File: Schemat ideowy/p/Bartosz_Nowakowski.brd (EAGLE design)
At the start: 41.6 x 33.5 mm, 23 parts, among them J2 6_PIN_SERIAL_CABLEPTH, U1 ESP8266, U2 4MB Flash, Y1 CRYSTAL-26MHZSMD-3.2X2.5

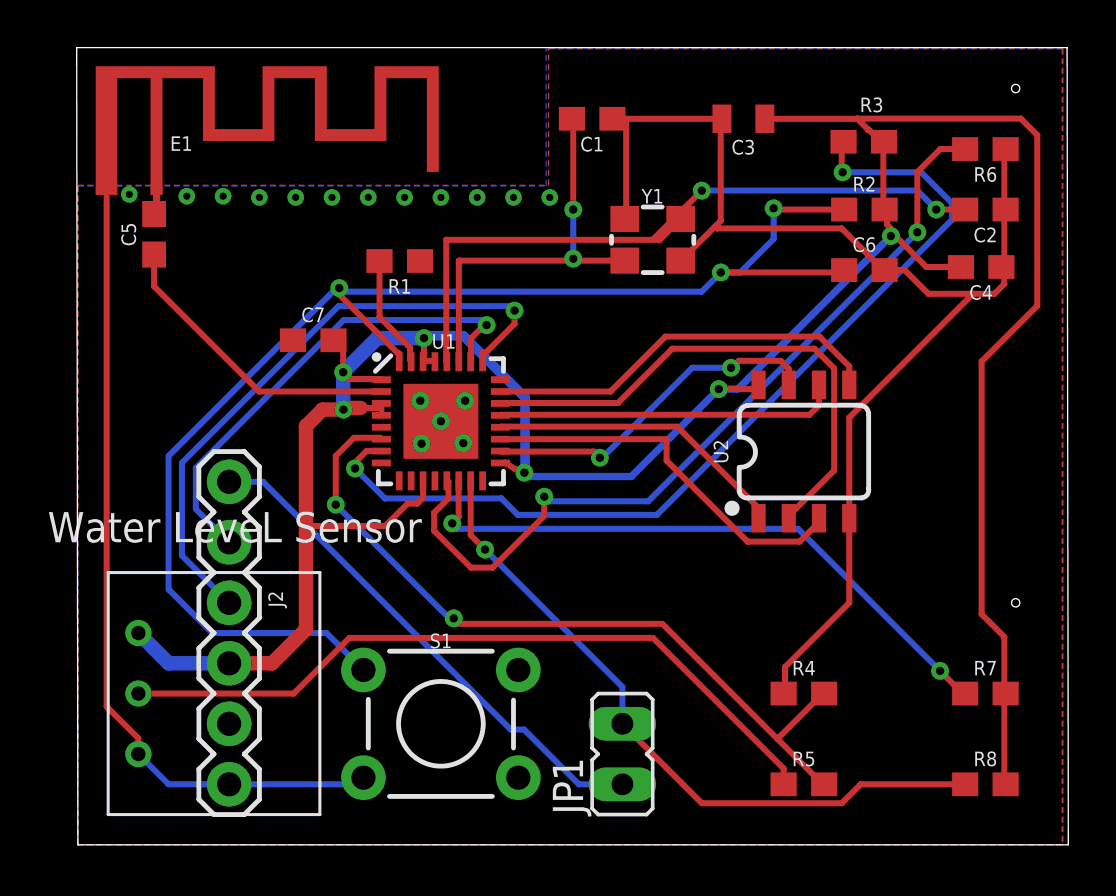
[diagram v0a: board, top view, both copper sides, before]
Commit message: update
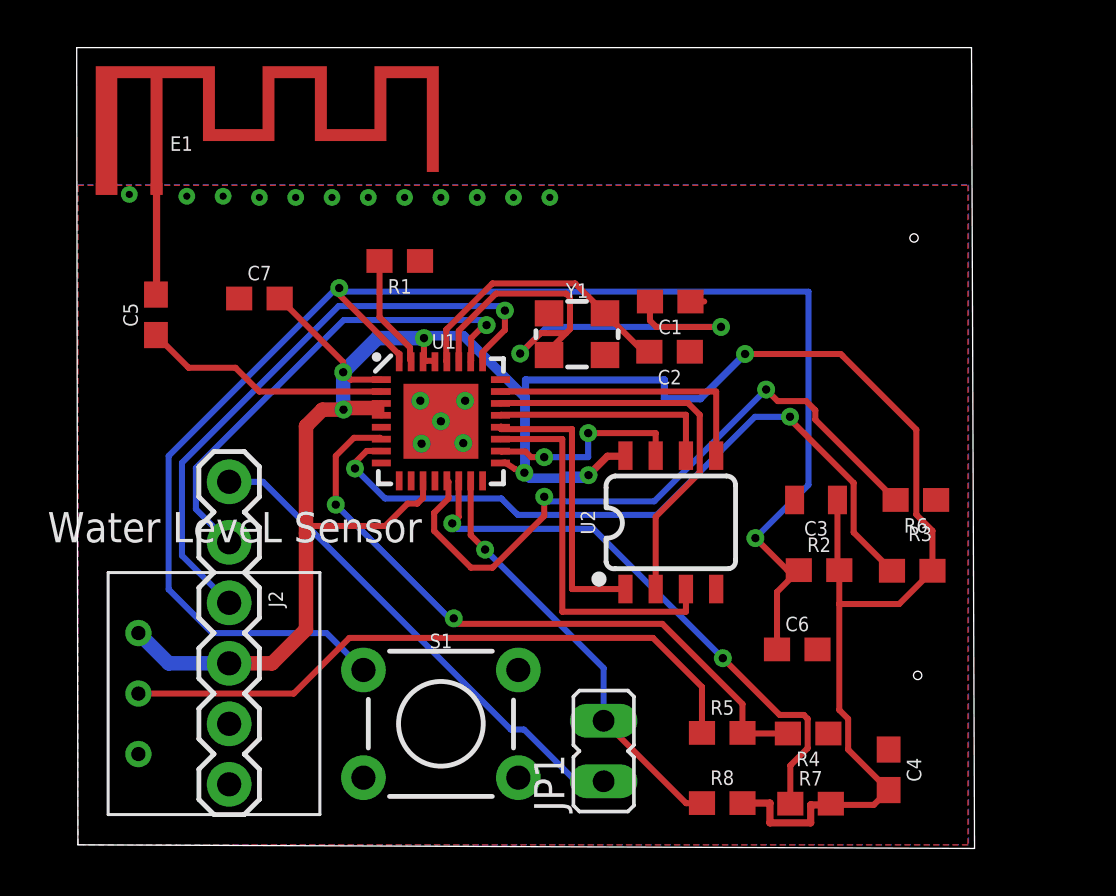
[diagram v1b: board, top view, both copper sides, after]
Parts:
- moved C4 21.5 mm to (34.0, 3.15), turned to 270 degrees
- moved R3 18.1 mm to (35.0, 11.5)
- moved C3 16.3 mm to (31.0, 14.5)
- moved C6 16.2 mm to (30.2, 8.20)
- moved R2 15.3 mm to (31.1, 11.5)
- moved R6 15.0 mm to (35.2, 14.5)
- moved C2 14.5 mm to (24.8, 20.7)
- moved R8 11.1 mm to (27.1, 1.75)
- moved R7 8.67 mm to (30.8, 1.73)
- moved C1 8.34 mm to (24.9, 22.8)
- moved U2 6.33 mm to (24.9, 13.5)
- moved Y1 5.08 mm to (21.0, 21.4)
- moved R5 4.05 mm to (27.1, 4.70)
- moved C5 3.38 mm to (3.28, 22.3)
- moved C7 2.86 mm to (7.62, 22.9)
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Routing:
- net GND: track 90.2 -> 1.39 mm
- net N$3: track 29.6 -> 11.9 mm, vias 2 -> 0
- net GPIO0: track 28.9 -> 18.0 mm
- net N$4: track 39.7 -> 30.6 mm
- net N$5: track 58.2 -> 66.6 mm, vias 3 -> 2
- net N$2: track 17.2 -> 24.5 mm
- net GPIO15: track 34.7 -> 28.3 mm
- net SD_HD: track 14.7 -> 8.58 mm
- net +3V3: track 118.4 -> 112.5 mm
- net SD_SO: track 22.4 -> 16.7 mm
- net SD_SI: track 16.9 -> 11.7 mm
- net SD_CLK: track 14.4 -> 9.51 mm
- net N$8: track 32.8 -> 28.4 mm
- net N$9: track 31.0 -> 27.4 mm
- net N$7: track 1.10 -> 4.45 mm
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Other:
- board size 41.6 x 33.5 mm -> 37.7 x 33.6 mm

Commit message: update
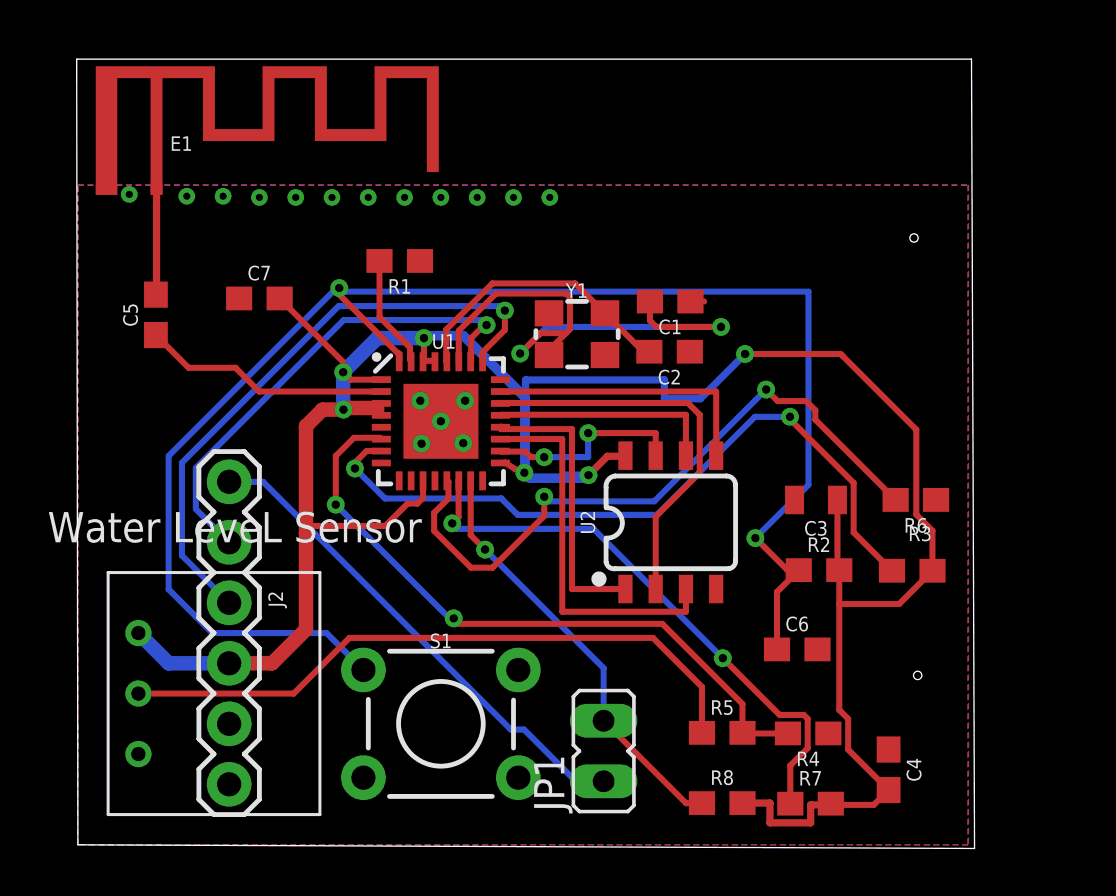
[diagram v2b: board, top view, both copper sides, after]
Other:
- board size 37.7 x 33.6 mm -> 37.7 x 33.1 mm
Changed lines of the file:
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@@
 <plain>
 <wire x1="0" y1="0" x2="37.643" y2="-0.1524" width="0" layer="20"/>
-<wire x1="37.643" y1="-0.1524" x2="37.516" y2="33.4672" width="0" layer="20"/>
-<wire x1="37.516" y1="33.4672" x2="-0.0508" y2="33.4672" width="0" layer="20"/>
-<wire x1="-0.0508" y1="33.4672" x2="0" y2="0" width="0" layer="20"/>
+<wire x1="37.643" y1="-0.1524" x2="37.516" y2="32.9846" width="0" layer="20"/>
+<wire x1="37.516" y1="32.9846" x2="-0.0508" y2="32.9846" width="0" layer="20"/>
+<wire x1="-0.0508" y1="32.9846" x2="0" y2="0" width="0" layer="20"/>
 <hole x="35.1028" y="25.4762" drill="0.35"/>
 <hole x="35.2552" y="7.112" drill="0.35"/>
